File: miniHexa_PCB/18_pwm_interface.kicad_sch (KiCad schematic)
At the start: 28 parts, among them U5 PCA9685BS

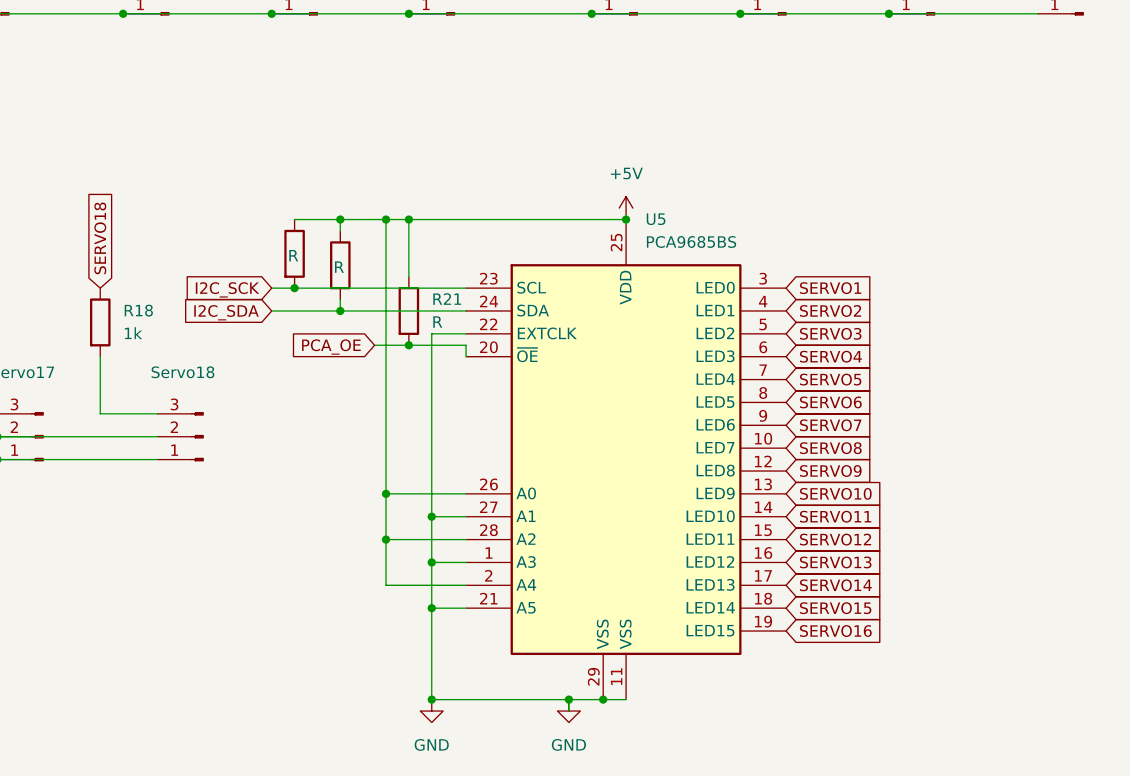
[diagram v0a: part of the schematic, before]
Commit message: update
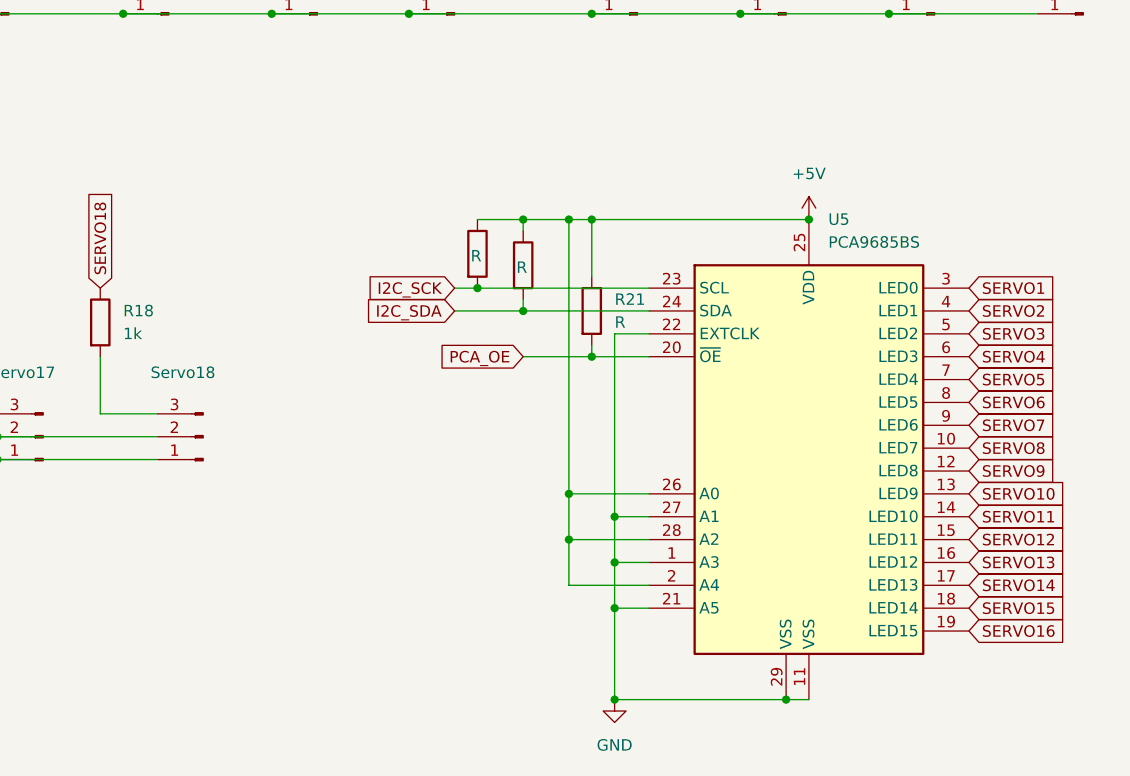
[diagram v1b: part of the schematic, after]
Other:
- moved on the sheet: R21, U5
